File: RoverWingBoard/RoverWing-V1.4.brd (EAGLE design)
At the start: 81.3 x 81.3 mm, 82 parts, among them CON1 XT30PW-M, J10 HEADER-PH-4P, J11 HEADER-PH-3P, J12 HEADER-3X04, J13 HEADER-3X06", J14 HEADER-2X16, J15 HEADER-2X12, J16 DF13-4P-1.25DSA, J17 DF13-6P-1.25DSA, J2 HEADER-VH, J3 HEADER-VH, J4 HEADER-PH-4P, J5 HEADER-PH-4P, J6 HEADER-PH-4P, J8 HEADER-PH-4P, J9 HEADER-PH-4P, SW1 SW-TACTILE-4.5X4.5_SMD, U1 ATSAMD21G, U2 MP2225, U3 PMIC-AZ1117EH-3.3, U5 DRV8871, U6 DRV8871, U7 TXS0104EPWR, U8 74AHCT1G125DBV, U9 ICM-42605

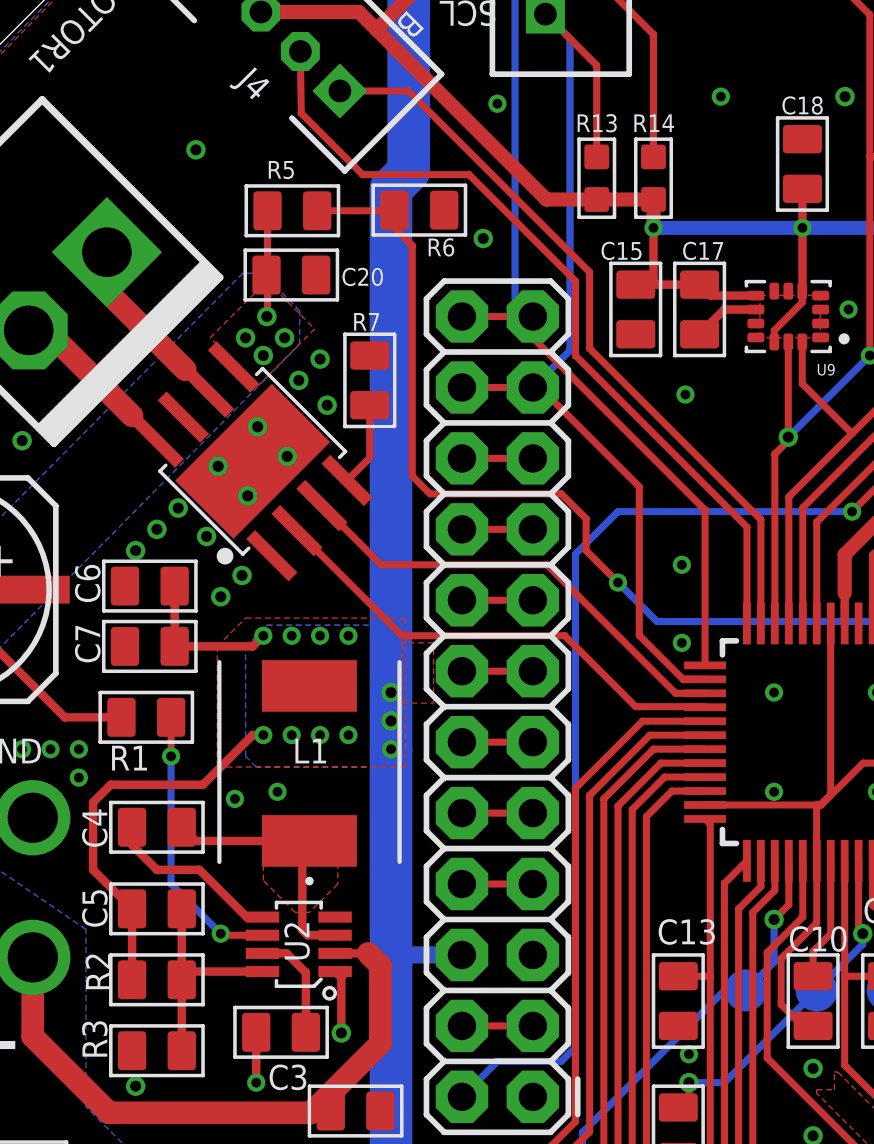
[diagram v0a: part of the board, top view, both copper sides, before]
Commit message: Update RoverWing-V1.4.brd
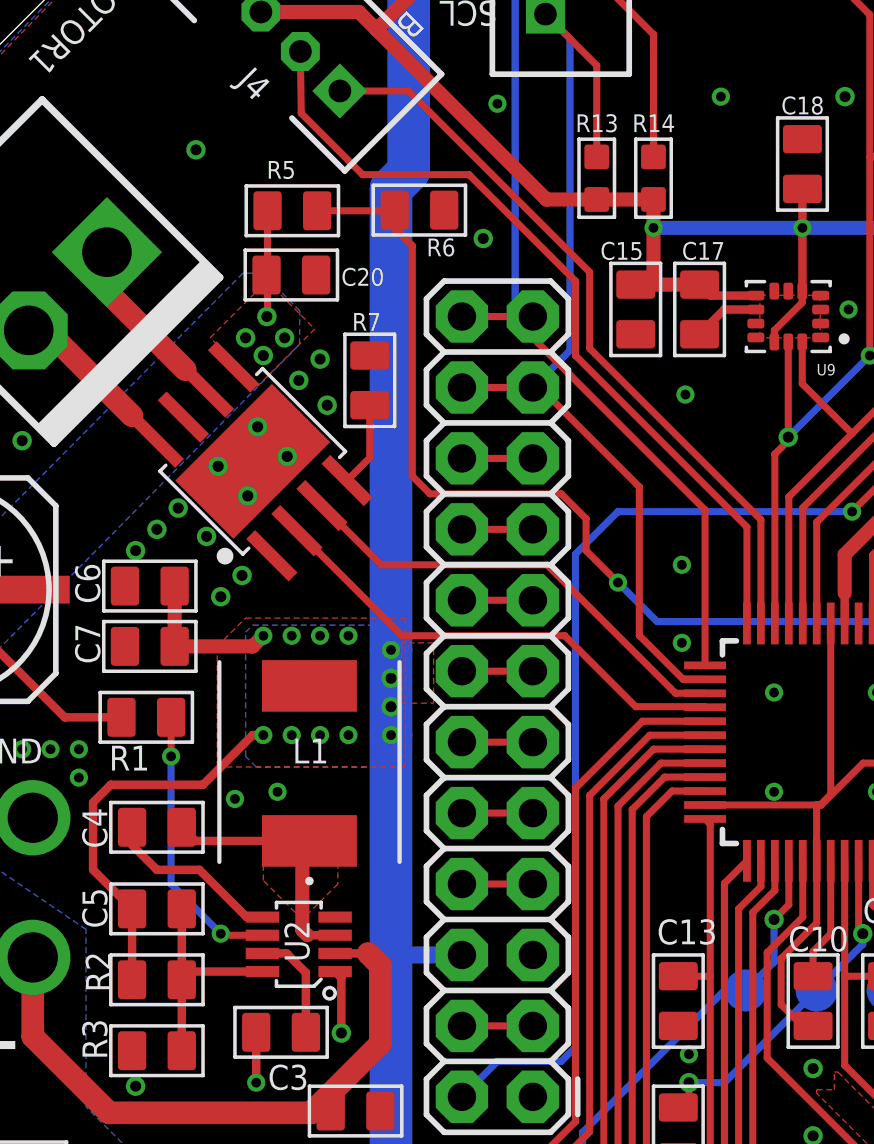
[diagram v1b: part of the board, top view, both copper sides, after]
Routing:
- net 5V: vias 16 -> 17
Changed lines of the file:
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@@
 <via x="-26.416" y="2.54" extent="1-16" drill="0.35"/>
 <via x="-27.432" y="3.556" extent="1-16" drill="0.35"/>
-<wire x1="-26.416" y1="3.556" x2="-27.432" y2="3.556" width="0" layer="19" extent="1-1"/>
 </signal>
 <signal name="3.3V">
@@
 <wire x1="-2.176" y1="19.8" x2="-3.798" y2="19.8" width="0.3048" layer="1"/>
 <wire x1="-3.798" y1="19.8" x2="-4.191" y2="20.193" width="0.3048" layer="1"/>
-<wire x1="-4.191" y1="20.193" x2="-5.969" y2="20.193" width="0.3048" layer="1"/>
+<wire x1="-4.191" y1="20.193" x2="-5.969" y2="20.193" width="0.508" layer="1"/>
 <wire x1="-5.969" y1="20.193" x2="-6.477" y2="20.193" width="0.3048" layer="1"/>
-<wire x1="-5.842" y1="22.225" x2="-5.842" y2="20.32" width="0.3048" layer="1"/>
+<wire x1="-5.842" y1="22.225" x2="-5.842" y2="20.32" width="0.508" layer="1"/>
 <wire x1="-5.842" y1="20.32" x2="-5.969" y2="20.193" width="0.3048" layer="1"/>
 <wire x1="-0.508" y1="23.622" x2="-0.508" y2="22.225" width="0.3048" layer="1"/>
@@
 <wire x1="-14.605" y1="33.909" x2="-10.033" y2="38.481" width="1.524" layer="16"/>
 <wire x1="-10.033" y1="38.481" x2="-4.064" y2="38.481" width="1.524" layer="16"/>
-<via x="-15.24" y="5.588" extent="1-16" drill="0.3937"/>
-<via x="-15.24" y="4.572" extent="1-16" drill="0.3937"/>
+<via x="-15.24" y="6.096" extent="1-16" drill="0.3937"/>
+<via x="-15.24" y="5.08" extent="1-16" drill="0.3937"/>
 <wire x1="-4.064" y1="38.481" x2="4.064" y2="38.481" width="1.524" layer="16"/>
 <wire x1="4.064" y1="38.481" x2="10.16" y2="38.481" width="1.524" layer="16"/>
@@
 <contactref element="J8" pad="3"/>
 <contactref element="R4" pad="2"/>
-<wire x1="-15.24" y1="-3.81" x2="-15.24" y2="3.556" width="1.524" layer="16"/>
-<wire x1="-15.24" y1="3.556" x2="-15.24" y2="23.622" width="1.524" layer="16"/>
+<wire x1="-15.24" y1="-3.81" x2="-15.24" y2="4.064" width="1.524" layer="16"/>
+<wire x1="-15.24" y1="4.064" x2="-15.24" y2="7.112" width="1.524" layer="16"/>
+<wire x1="-15.24" y1="7.112" x2="-15.24" y2="23.622" width="1.524" layer="16"/>
 <wire x1="-15.24" y1="23.622" x2="-14.605" y2="24.257" width="1.524" layer="16"/>
 <wire x1="-14.605" y1="24.257" x2="-14.605" y2="33.909" width="1.524" layer="16"/>
@@
 <vertex x="-14.730290625" y="2.921"/>
 </polygon>
-<via x="-15.24" y="3.556" extent="1-16" drill="0.35"/>
+<via x="-15.24" y="4.064" extent="1-16" drill="0.35"/>
 <polygon width="0.0254" layer="16" thermals="no">
 <vertex x="-14.732" y="2.921"/>
 <vertex x="-20.066" y="2.921"/>
 <vertex x="-20.447" y="3.302"/>
-<vertex x="-20.447" y="7.239"/>
-<vertex x="-19.685" y="8.001"/>
+<vertex x="-20.447" y="7.747"/>
+<vertex x="-20.193" y="8.001"/>
 <vertex x="-15.494" y="8.001"/>
 <vertex x="-14.732" y="7.239"/>
@@
 <wire x1="31.279196875" y1="17.373378125" x2="31.279196875" y2="14.861403125" width="0.508" layer="1"/>
 <wire x1="15.24" y1="28.194" x2="17.8435" y2="30.7975" width="0.508" layer="16"/>
-<wire x1="-22.987" y1="9.398" x2="-22.987" y2="7.239" width="0.3048" layer="1"/>
-<wire x1="-20.193" y1="7.239" x2="-19.812" y2="7.62" width="0.3048" layer="1"/>
-<wire x1="-22.987" y1="7.239" x2="-20.193" y2="7.239" width="0.3048" layer="1"/>
+<wire x1="-22.987" y1="9.398" x2="-22.987" y2="7.239" width="0.508" layer="1"/>
+<wire x1="-20.193" y1="7.239" x2="-19.812" y2="7.62" width="0.508" layer="1"/>
+<wire x1="-22.987" y1="7.239" x2="-20.193" y2="7.239" width="0.508" layer="1"/>
 <wire x1="-15.24" y1="-11.43" x2="-22.225" y2="-11.43" width="0.3048" layer="16"/>
 <wire x1="-22.225" y1="-11.43" x2="-22.352" y2="-11.43" width="0.3048" layer="16"/>
@@
 <wire x1="-22.225" y1="-11.43" x2="-22.257" y2="-11.398" width="0.3048" layer="1"/>
 <wire x1="-22.257" y1="-11.398" x2="-27.619" y2="-11.398" width="0.3048" layer="1"/>
+<via x="-15.24" y="7.112" extent="1-16" drill="0.35"/>
 <wire x1="2.286" y1="-31.75" x2="2.286" y2="-31.623" width="0" layer="19" extent="16-16"/>
 <wire x1="0.9144" y1="-30.2514" x2="1.0795" y2="-30.5435" width="0" layer="19" extent="1-16"/>
@@
 <contactref element="C4" pad="2"/>
 <wire x1="-17.242" y1="-3.104" x2="-18.232" y2="-3.104" width="0.3048" layer="1"/>
-<wire x1="-18.232" y1="-3.104" x2="-18.415" y2="-2.921" width="0.3048" layer="1"/>
+<wire x1="-18.232" y1="-3.104" x2="-18.415" y2="-2.921" width="0.508" layer="1"/>
 <wire x1="-18.1102" y1="0.0561375" x2="-18.1102" y2="0.273" width="0.3048" layer="1"/>
-<wire x1="-18.415" y1="-2.921" x2="-18.415" y2="-0.2486625" width="0.3048" layer="1"/>
+<wire x1="-18.415" y1="-2.921" x2="-18.415" y2="-0.2486625" width="0.508" layer="1"/>
 <wire x1="-18.415" y1="-0.2486625" x2="-18.1102" y2="0.0561375" width="0.3048" layer="1"/>
 <wire x1="-18.161" y1="0.273" x2="-22.244" y2="0.273" width="0.3048" layer="1"/>
